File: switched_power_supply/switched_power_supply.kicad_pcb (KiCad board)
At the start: 2 copper layers, 80 x 60 mm, 36 parts, among them IC1 VIPER53ESPTR-E, T1 Transformador_1x2, U1 Viper53, U2 TL431, U3 PC817 Opto

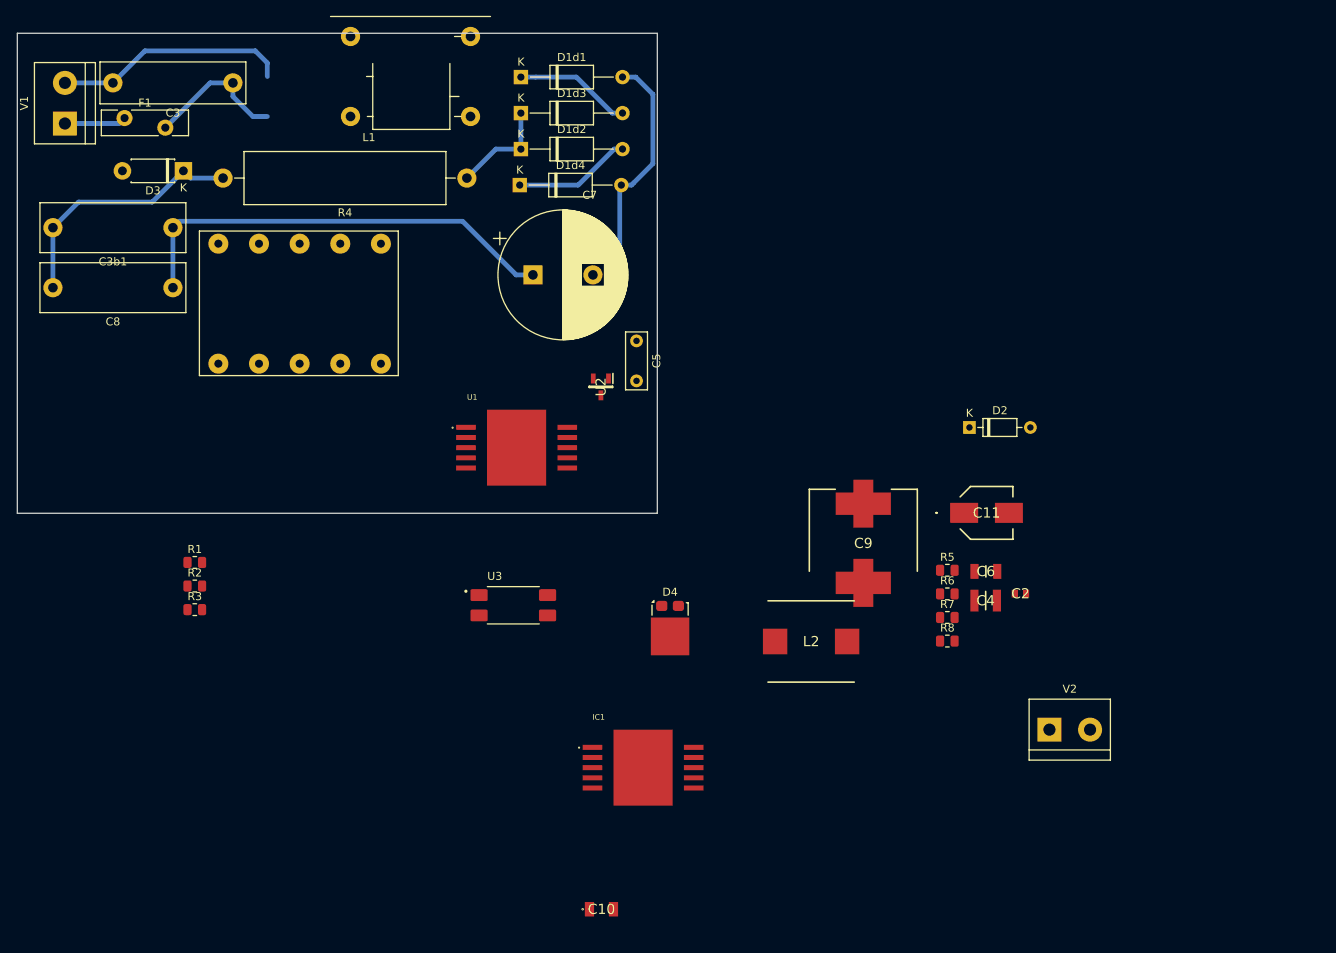
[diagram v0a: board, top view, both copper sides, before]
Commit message: Uploading files
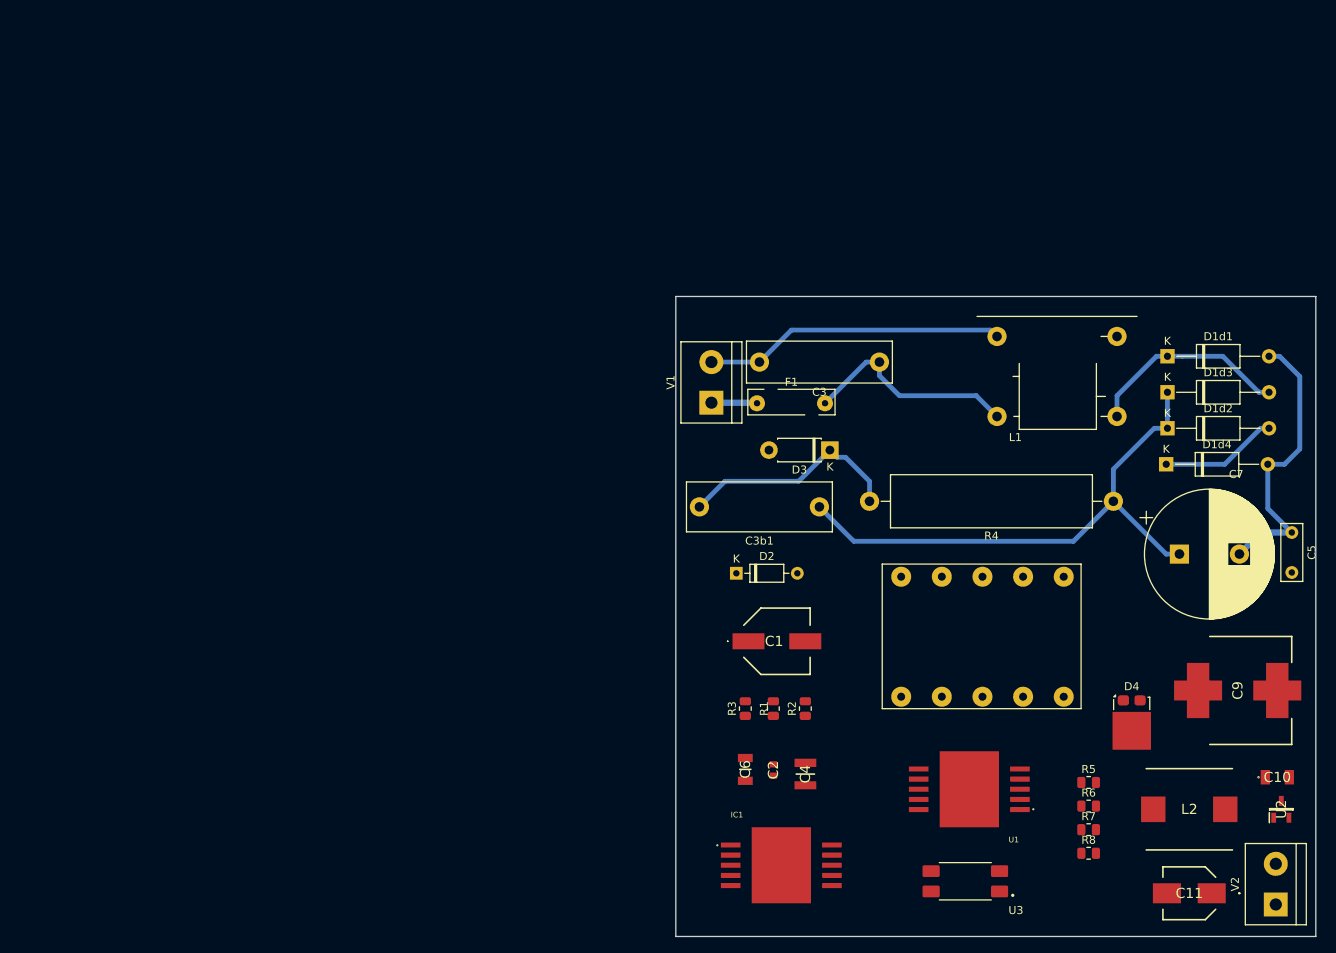
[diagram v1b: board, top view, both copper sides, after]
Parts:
- removed C8: Capacitor_Filme, Capacitor_THT:C_Rect_L18.0mm_W6.0mm_P15.00mm_FKS3_FKP3
- added C1: Capacitor_Eletrolitico, pci:EEHZT1E331UP, F.Cu at (119.5, 96.0)
- moved U2 100.1 mm to (182.5, 117.0), turned to 90 degrees
- moved T1 95.0 mm to (132.6, 104.6)
- moved R4 90.3 mm to (161.5, 78.5)
- moved L1 89.1 mm to (162.0, 67.9)
- moved D1d4 88.0 mm to (168.1, 73.9)
- moved C3b1 88.0 mm to (124.8, 79.2)
- moved D3 88.0 mm to (126.1, 72.1)
- moved F1 88.0 mm to (118.7, 65.5)
- moved V1 88.0 mm to (111.3, 66.2)
- moved C3 88.0 mm to (132.3, 61.1)
- moved C7 88.0 mm to (169.8, 85.1)
- moved D1d1 88.0 mm to (168.3, 60.4)
- moved D1d2 88.0 mm to (168.3, 69.4)
- moved D1d3 88.0 mm to (168.3, 64.9)
- moved C10 86.1 mm to (182.0, 113.0)
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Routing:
- net Net-(D1d1-K): track 14.6 -> 25.5 mm
- net Net-(C3-Pad1): track 17.8 -> 27.4 mm
- net Net-(C3-Pad2): track 29.3 -> 37.7 mm
- net GND: track 29.3 -> 36.8 mm
- net Net-(D3-K): track 32.1 -> 28.3 mm
- net Net-(F1-Pad1): track 7.73 -> 5.73 mm
- net /BarP: track 68.4 -> 70.1 mm
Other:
- board size 80 x 60 mm -> 80 x 80 mm
